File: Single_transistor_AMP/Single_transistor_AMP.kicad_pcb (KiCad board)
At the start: 4 copper layers, 0 parts

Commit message: 6nod md
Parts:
- added 100ohm1: R5, Resistor_SMD:R_0402_1005Metric, F.Cu at (143.1, 113.4)
- added C1: 0,1uF, Capacitor_SMD:C_0402_1005Metric, F.Cu at (143.1, 116.3)
- added C2: 0,1uF, Capacitor_SMD:C_0402_1005Metric, F.Cu at (145.8, 113.4)
- added C3: 0,1uF, Capacitor_SMD:C_0402_1005Metric, F.Cu at (158.8, 112.3)
- added J1: Screw_Terminal_01x02, TerminalBlock_MetzConnect:TerminalBlock_MetzConnect_Type101_RT01602HBWC_1x02_P5.08mm_Horizontal, F.Cu at (138.8, 105.0)
- added J2: Screw_Terminal_01x02, TerminalBlock_MetzConnect:TerminalBlock_MetzConnect_Type101_RT01602HBWC_1x02_P5.08mm_Horizontal, F.Cu at (151.2, 105.0)
- added Q1: 2N2222A, Package_TO_SOT_THT:TO-92_Inline, F.Cu at (138.3, 115.5)
- added Q2: 2N2222A, Package_TO_SOT_THT:TO-92_Inline, F.Cu at (154.6, 115.4)
- added R1: 1kohm, Resistor_SMD:R_0402_1005Metric, F.Cu at (149.5, 112.9)
- added R2: 20kohm, Resistor_SMD:R_0402_1005Metric, F.Cu at (148.5, 116.5)
- added R3: 1kohm, Resistor_SMD:R_0402_1005Metric, F.Cu at (158.7, 115.4)
- added R4: 3kohm, Resistor_SMD:R_0402_1005Metric, F.Cu at (145.9, 116.2)
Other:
- board outline added: 28.1 x 19.4 mm

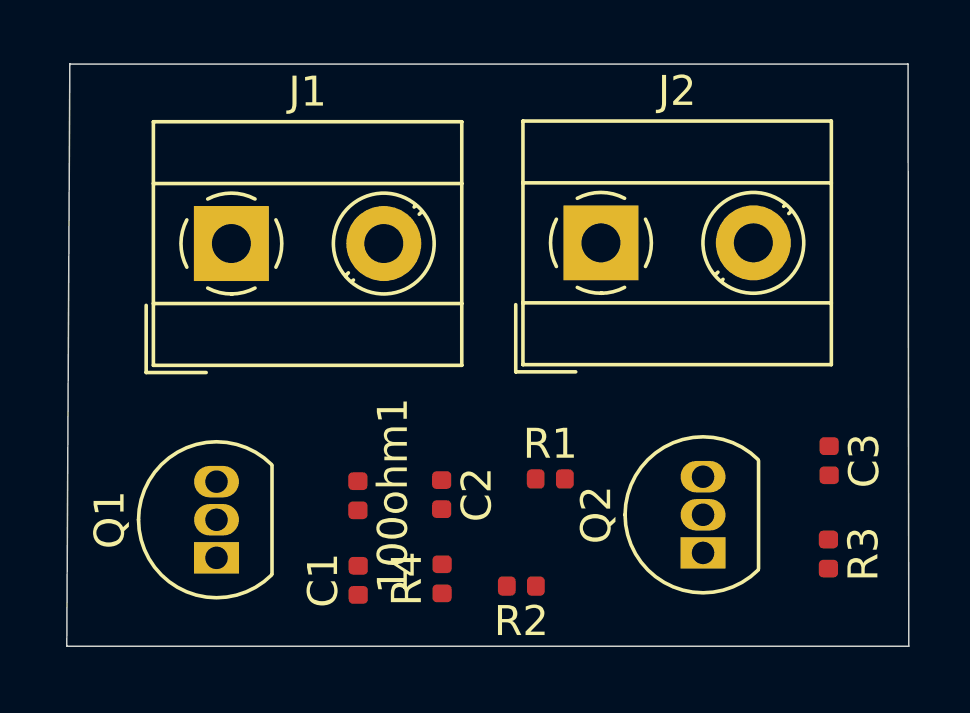
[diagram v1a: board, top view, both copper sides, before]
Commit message: md
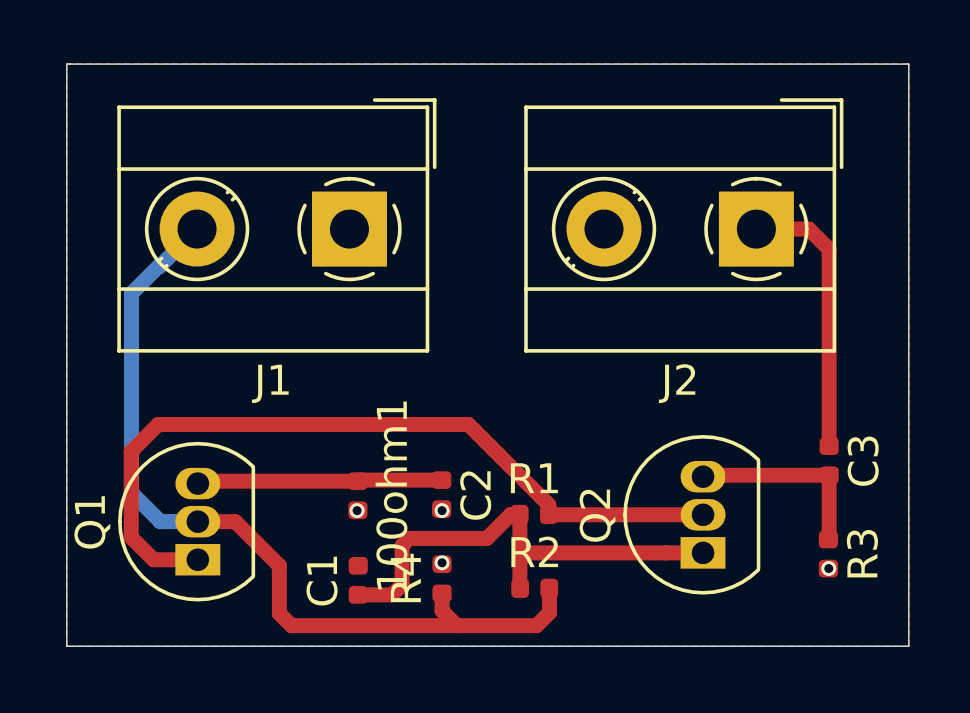
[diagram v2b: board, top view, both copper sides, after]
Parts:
- moved J2 5.20 mm to (156.3, 104.6), turned to 180 degrees
- moved J1 3.97 mm to (142.8, 104.6), turned to 180 degrees
- moved R1 1.30 mm to (148.9, 114.1)
- moved Q1 0.63 mm to (137.7, 115.6)
- moved R2 0.45 mm to (148.9, 116.5), turned to 0 degrees
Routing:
- net Net-(J1-Pad2): track 0.00 -> 28.7 mm
- net Net-(Q1-Pad1): track 0.00 -> 26.3 mm
- net +15V: track 0.00 -> 15.8 mm
- net Net-(C3-Pad1): track 0.00 -> 9.27 mm
- net Net-(100ohm1-Pad1): track 0.00 -> 8.18 mm
- net Net-(C3-Pad2): track 0.00 -> 6.38 mm
- net GNDREF: vias 0 -> 4
- added copper zone on B.Cu, net GNDREF
- added copper zone on F.Cu, net GNDREF
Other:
- outline, holes or cut-outs redrawn
